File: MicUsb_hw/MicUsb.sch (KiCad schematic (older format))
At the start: 52 parts, among them Q1 DVIUC6-4SC6

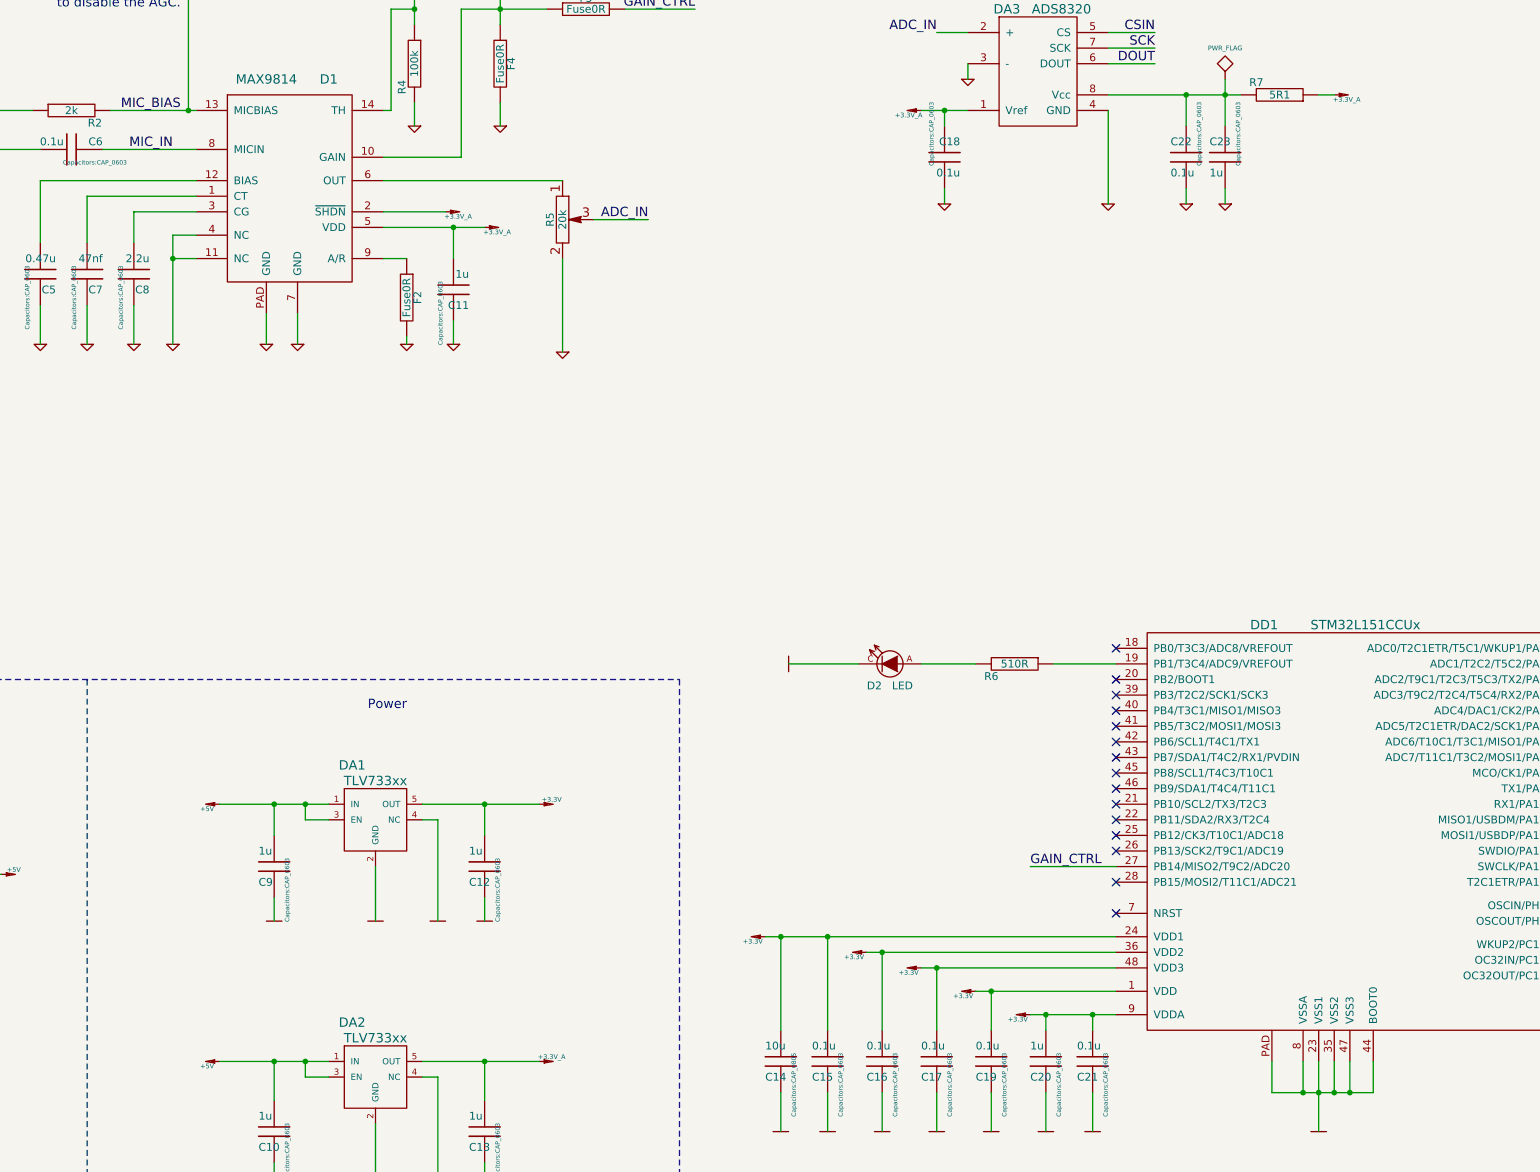
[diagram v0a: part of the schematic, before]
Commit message: small scheme updates
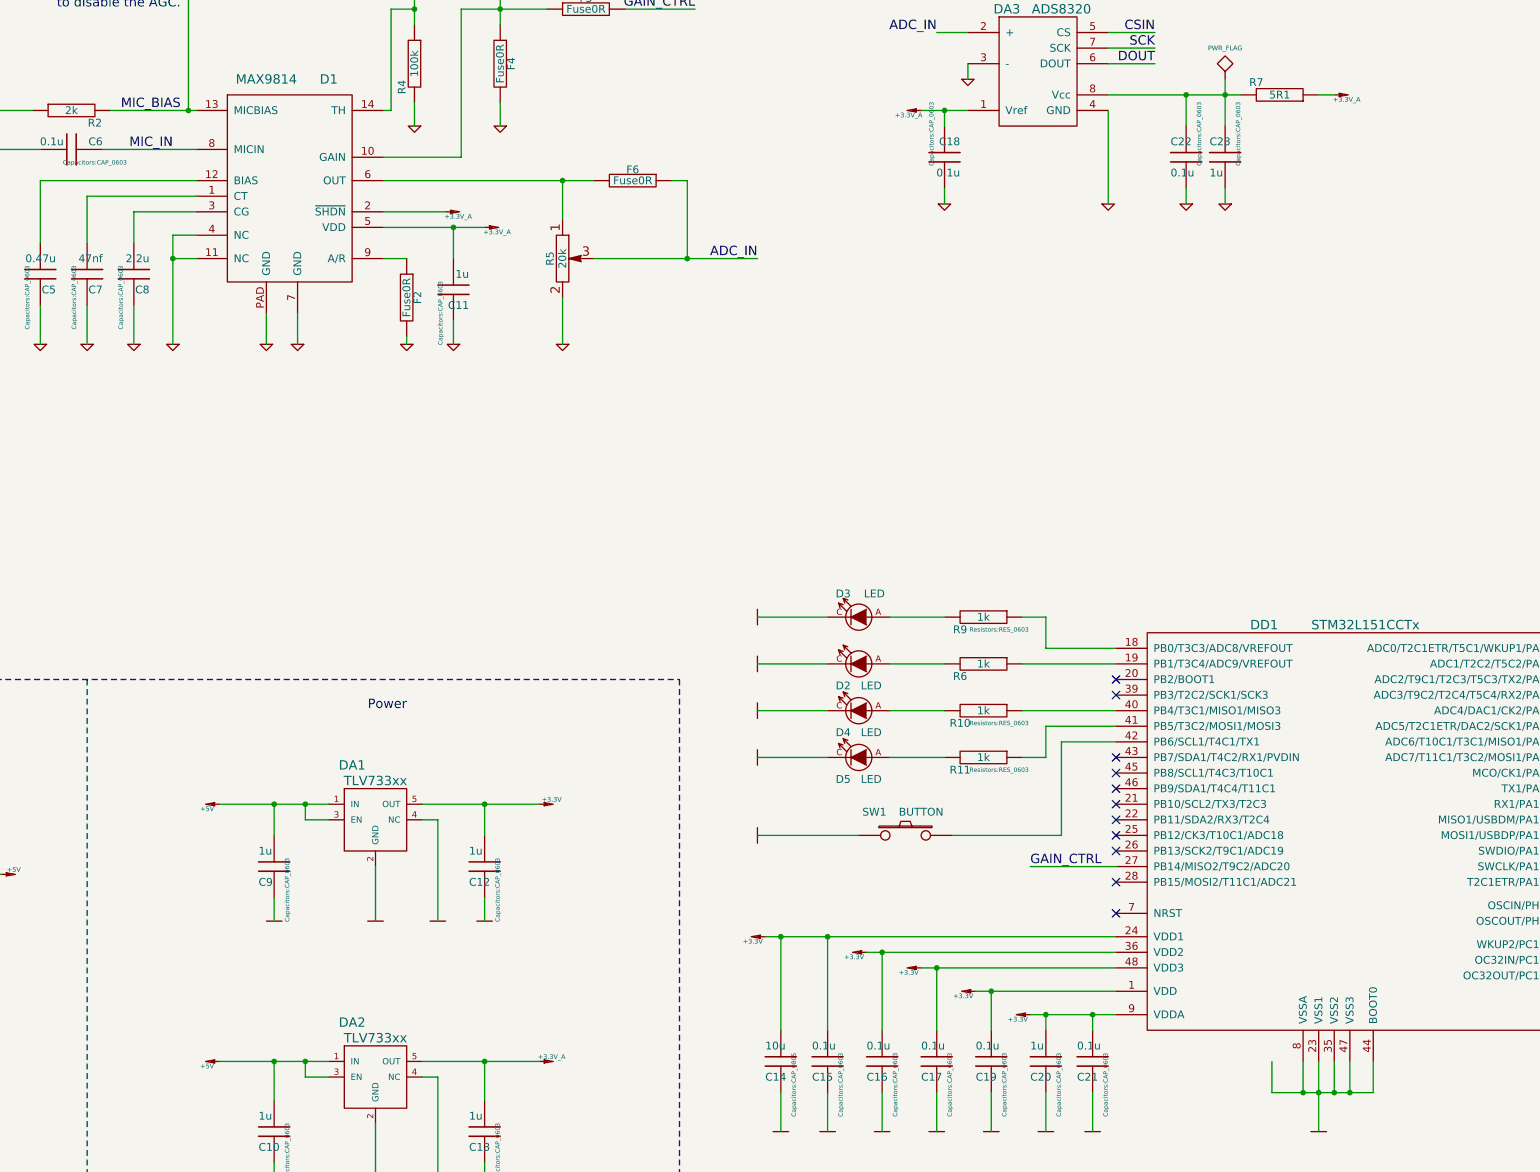
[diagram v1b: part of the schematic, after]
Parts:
- removed DD1: STM32L151CCUx, symbol STM32L151CCUx
- added D3, D4, D5: LED, LEDs:LED_0603, symbol LED
- added DD1: STM32L151CCTx, LQFP_TQFP:LQFP48, symbol STM32L151CCTx
- added F6: Fuse0R, Resistors:RES_0603_SOLDERFUSE, symbol Fuse0R
- added R10, R11, R9: 1k, Resistors:RES_0603, symbol R
- added SW1: BUTTON, BtnsSwitches:BTN_6x6, symbol BUTTON
- DA3: footprint (none) -> SO_DIL_TSSOP:MSOP8
- R6: value 510R -> 1k
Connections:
- net +3.3V: now also DD1.1 (VDD), DD1.24 (VDD1), DD1.36 (VDD2), DD1.48 (VDD3), DD1.9 (VDDA)
- net ADC_IN: now also F6.1
- net CSIN: now also DD1.14 (ADC4/DAC1/CK2/PA4)
- net D+: now also DD1.33 (MOSI1/USBDP/PA12)
- net D-: now also DD1.32 (MISO1/USBDM/PA11)
- net DOUT: now also DD1.16 (ADC6/T10C1/T3C1/MISO1/PA6)
- net GAIN_CTRL: now also DD1.27 (PB14/MISO2/T9C2/ADC20)
- net GND: now also D3.C, D4.C, D5.C, DD1.23 (VSS1), DD1.35 (VSS2), DD1.44 (BOOT0), DD1.47 (VSS3), DD1.8 (VSSA), SW1.1
- net RX: now also DD1.31 (RX1/PA10)
- net SCK: now also DD1.15 (ADC5/T2C1ETR/DAC2/SCK1/PA5)
- net SWCLK: now also DD1.37 (SWCLK/PA14)
- net SWDIO: now also DD1.34 (SWDIO/PA13)
- net TX: now also DD1.30 (TX1/PA9)
- net at R6.1: now also DD1.19 (PB1/T3C4/ADC9/VREFOUT)
- net at C25.1, XTAL1.2: now also DD1.5 (OSCIN/PH0)
- net at R8.2: now also DD1.6 (OSCOUT/PH1)
- net at D1.6 (OUT), R5.1: now also F6.2
- new net: DD1.18 (PB0/T3C3/ADC8/VREFOUT), R9.1
- new net: D3.A, R9.2
- new net: DD1.40 (PB4/T3C1/MISO1/MISO3), R10.1
- new net: D4.A, R10.2
- new net: DD1.41 (PB5/T3C2/MOSI1/MOSI3), R11.1
- new net: D5.A, R11.2
- new net: DD1.42 (PB6/SCL1/T4C1/TX1), SW1.2
- no-connect marks 26 -> 22
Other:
- moved on the sheet: D2, R5, R6

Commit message: + LP filter, i need answers!
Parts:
- added C? (x3): 1n, CAP_0603, symbol C
- added C?: 1.8n, CAP_0603, symbol C
- added C?: 12n, CAP_0603, symbol C
- added C?: 47n, CAP_0603, symbol C
- added C?: 10n, CAP_0603, symbol C
- added C?: 4.7u, CAP_0603, symbol C
- added DA? (x4): Generic_14pin, symbol Generic_14pin
- added R?: 75k, RES_0603, symbol R
- added R?: 39k, RES_0603, symbol R
- added R?: 9.1k, RES_0603, symbol R
- added R?: 15k, RES_0603, symbol R
- added R?: 3k, RES_0603, symbol R
- added R?: 4.7k, RES_0603, symbol R
- added R?: 75R, RES_0603, symbol R
- added R?: 120R, RES_0603, symbol R
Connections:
- net +3.3V_A: now also DA?.4 (V+), DA?.4 (V+), DA?.4 (V+), DA?.4 (V+)
- net AGND: now also C?.2, C?.2, C?.2, C?.2, DA?.11 (V-), DA?.11 (V-), DA?.11 (V-), DA?.11 (V-)
- new net: C?.1, DA?.1, DA?.2 (-), R?.2 (x3)
- new net: C?.1, DA?.3 (+), R?.1 (x4)
- new net: C?.2, R?.1, R?.2 (x4)
- new net: C?.1, DA?.1, DA?.2 (-)
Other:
- moved on the sheet: C10, C11, C12, C13, C14, C15, C16, C17, C18, C19, C20, C21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
